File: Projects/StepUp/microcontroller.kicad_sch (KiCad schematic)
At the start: 31 parts, among them J1 USB_C_Receptacle_USB2.0_16P, J2 Conn_01x09_Pin, J3 Conn_02x03_Odd_Even, SW1 PTS636SP43SMTRL FS, SW2 PTS636SP43SMTRL FS, U1 W25Q16JVUXIQ TR, U2 USBLC6-2SC6, U3 RP2040, Y1 ABM8-272-T3

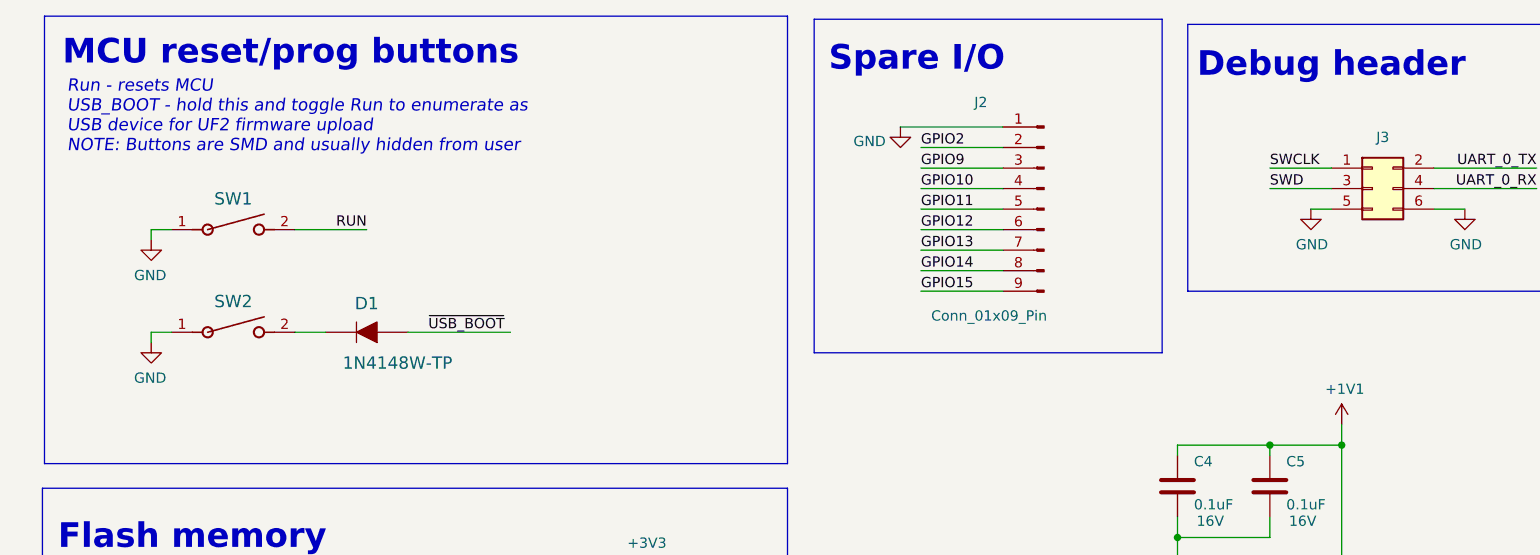
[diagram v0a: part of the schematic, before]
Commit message: feat(v0.3): Layout 90% complete
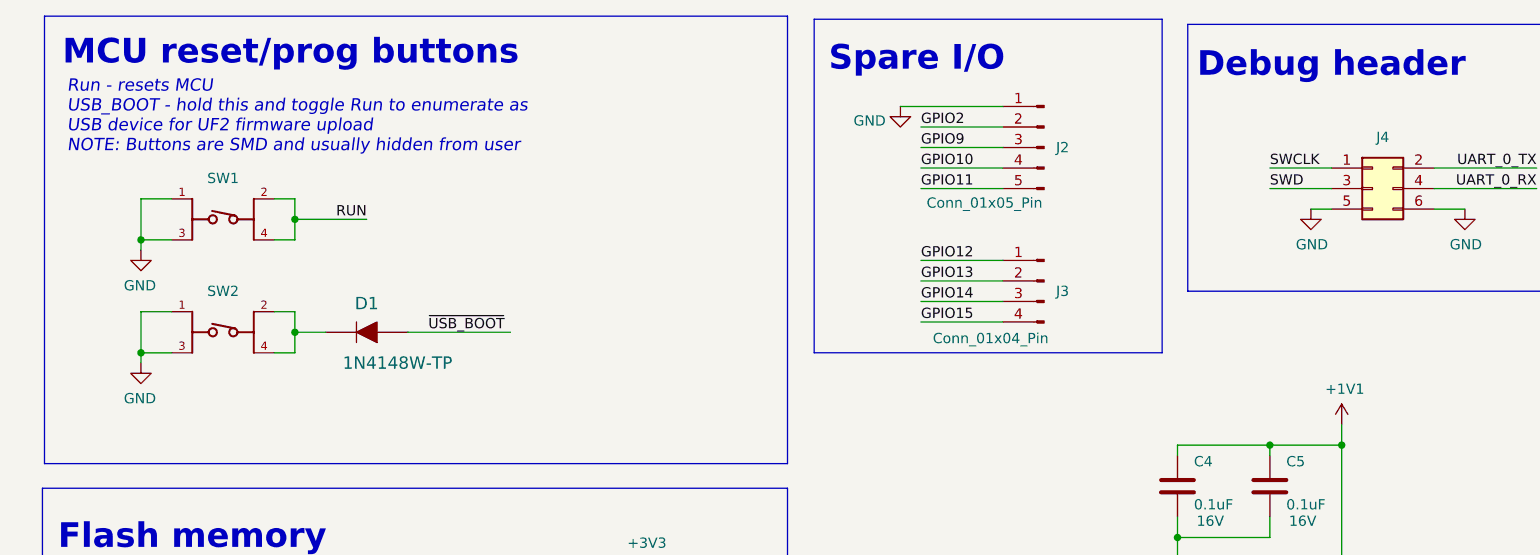
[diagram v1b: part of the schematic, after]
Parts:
- removed J2: Conn_01x09_Pin, Connector_PinHeader_2.54mm:PinHeader_1x09_P2.54mm_Vertical, symbol Connector:Conn_01x09_Pin
- removed SW1, SW2: PTS636SP43SMTRL FS, Snapeda:SW_PTS636S-J_CNK, symbol Snapeda_kicad:PTS636SL43SMTRLFS
- added J2: Conn_01x05_Pin, Connector_PinHeader_2.54mm:PinHeader_1x05_P2.54mm_Vertical, symbol Connector:Conn_01x05_Pin
- added J3: Conn_01x04_Pin, Connector_PinHeader_2.54mm:PinHeader_1x04_P2.54mm_Vertical, symbol Connector:Conn_01x04_Pin
- added SW1, SW2: 434153017835, Snapeda:434153017835_434153017835, symbol Snapeda:434153017835
- renumbered J3 to J4
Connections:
- net GND: now also J2.1 (Pin_1), SW1.1, SW1.3, SW2.1, SW2.3
- net GPIO10: now also J2.4 (Pin_4)
- net GPIO11: now also J2.5 (Pin_5)
- net GPIO12: now also J3.1 (Pin_1)
- net GPIO13: now also J3.2 (Pin_2)
- net GPIO14: now also J3.3 (Pin_3)
- net GPIO15: now also J3.4 (Pin_4)
- net GPIO2: now also J2.2 (Pin_2)
- net GPIO9: now also J2.3 (Pin_3)
- net RUN: now also SW1.2, SW1.4
- net at D1.K: now also SW2.2, SW2.4

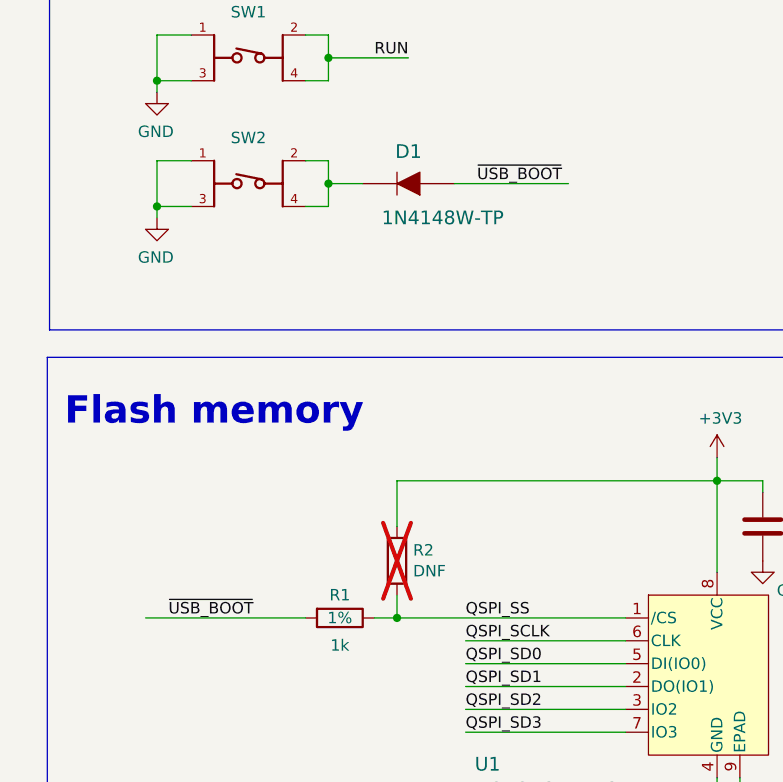
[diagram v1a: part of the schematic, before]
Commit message: feat(v0.3): Files sent to PCBWay for build
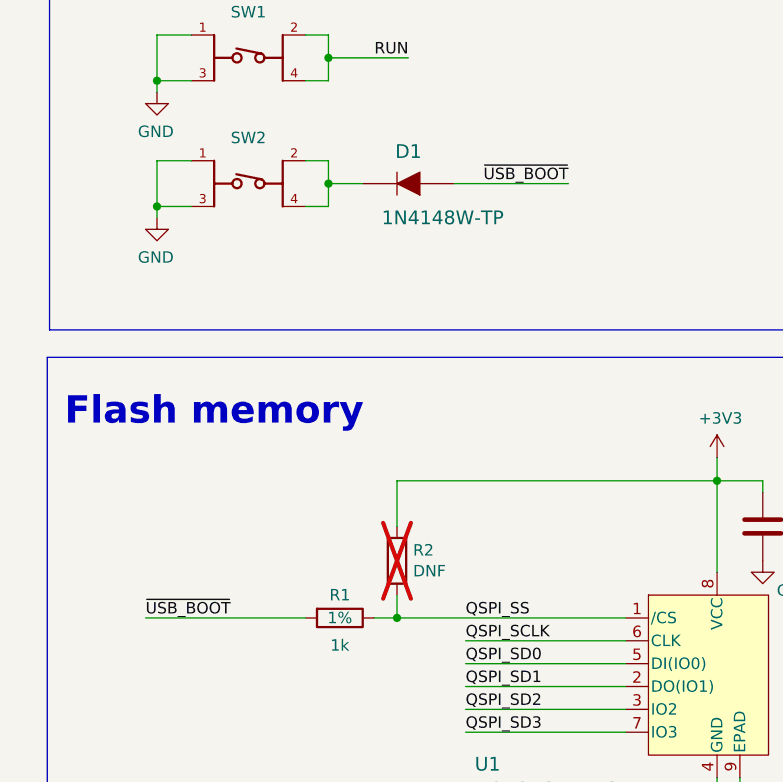
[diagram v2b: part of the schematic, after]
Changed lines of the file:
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@@
+			"AAAAAAAAAAAAAAAAAAAAAAAAAAAAAAAAAAAAAAAAAAAAAAAAAAAAAAAAAAAAAAAAAAAAAAAAAAAA"
+			"AAAAAAAAAAAAAAAAAAAAAAAAAAAAAAAAAAAAAAAAAAAAAAAAAAAAAAAAAAAAAAAAAAAAAAAAAAAA"
+			"AAAAAAAAAAAAAAAAAAAAAAAAAAAAAAAAAAAAAAAAAAAAAAAAAAAAAAAAAAAAAAAAAAAAAAAAAAAA"
+			"AAAAAAAAAAAAAAAAAAAAAAAAAAAAAAAAAAAAAAAAAAAAAAAAAAAAAAAAAAAAAAAAAAAAAAAAAAAA"
+			"AAAAAAAAAAAAAAAAAAAAAAAAAAAAAAAAAAAAAAAAAAAAAAAAAAAAAAAAAAAAAAAAAAAAAAAAAAAA"
+			"AAAAAAAAAAAAAAAAAAAAAAAAAAAAAAAAAAAAAAAAAAAAAAAAAAAAAAAAAAAAAAAAAAAAAAAAAAAA"
+			"AAAAAAAAAAAAAAAAAAAAAAAAAAAAAAAAAAAAAAAAAAAAAAAAAAAAAAAAAAAAAAAAAAAAAAAAAAAA"
+			"AAAAAAAAAAAAAAAAAAAAAAAAAAAAAAAAAAAAAAAAAAAAAAAAAAAAAAAAAAAAAAAAAAAAAAAAAAAA"
+			"AAAAAAAAAAAAAAAAAAAAAAAAAAAAAAAAAAAAAAAAAAAAAAAAAAAAAAAAAAAAAAAAAAAAAAAAAAAA"
+			"AAAAAAAAAAAAAAAAAAAAAAAAAAAAAAAAAAAAAAAAAAAAAAAAAAAAAAAAAAAAAAAAAAAAAAAAAAAA"
+			"AAAAAAAAAAAAAAAAAAAAAAAAAAAAAAAAAAAAAAAAAAAAAAAAAAAAAAAAAAAAAAAAAAAAAAAAAAAA"
+			"AAAAAAAAAAAAAAAAAAAAAAAAAAAAAAAAAAAAAAAAAAAAAAAAAAAAAAAAAAAAAAAAAAAAAAAAAAAA"
+			"AAAAAAAAAAAAAAAAAAAAAAAAAAAAAAAAAAAAAAAAAAAAAAAAAAAAAAAAAAAAAAAAAAAAAAAAAAAA"
+			"AAAAAAAAAAAAAAAAAAAAAAAAAAAAAAAAAAAAAAAAAAAAAAAAAAAAAAAAAAAAAAAAAAAAAAAAAAAA"
+			"AAAAAAAAAAAAAAAAAAAAAAAAAAAAAAAAAAAAAAAAAAAAAAAAAAAAAAAAAAAAAAAAAAAAAAAAAAAA"
+			"AAAAAAAAAAAAAAAAAAAAAAAAAAAAAAAAAAAAAAAAAAAAAAAAAAAAAAAAAAAAAAAAAAAAAAAAAAAA"
+			"AAAAAAAAAAAAAAAAAAAAAAAAAAAAAAAAAAAAAAAAAAAAAAAAAAAAAAAAAAAAAAAAAAAAAAAAAAAA"
+			"AAAAAAAAAAAAAAAAAAAAAAAAAAAAAAAAAAAAAAAAAAAAAAAAAAAAAAAAAAAAAAAAAAAAAAAAAAAA"
 			"AAAAAAAAAAAAAAAAAAAAAAAAAAAAAAAAAAAAAAAAAAAAAAAAAAAAAAAAAAAAAAAAAAAAAAAAAAAA"
 			"AAAAAAAAAAAAAAAAAAAAAAAAAAAAAAAAAAAAAAAAAAAAAAAAAAAAAAAAAAAAAAAAAAAAAAAAAAAA"
@@
 		)
 	)
+	(label "~{USB_BOOT}"
+		(at 43.18 114.3 0)
+		(effects
+			(font
+				(size 1.27 1.27)
+			)
+			(justify left bottom)
+		)
+	)
 	(label "UART_0_RX"
 		(at 217.17 48.26 180)
@@
 		)
 	)
+	(label "~{USB_BOOT}"
+		(at 90.17 66.04 180)
+		(effects
+			(font
+				(size 1.27 1.27)
+			)
+			(justify right bottom)
+		)
+	)
 	(label "GPIO12"
 		(at 140.97 57.15 0)
@@
 		)
 	)
-	(label "~{USB_BOOT}"
-		(at 45.72 114.3 0)
-		(effects
-			(font
-				(size 1.27 1.27)
-			)
-			(justify left bottom)
-		)
-	)
 	(label "GPIO15"
 		(at 140.97 64.77 0)
@@
 		(effects
 			(font
-				(size 1.27 1.27)
-			)
-			(justify left bottom)
-		)
-	)
-	(label "~{USB_BOOT}"
-		(at 80.01 66.04 0)
-		(effects
-			(font
